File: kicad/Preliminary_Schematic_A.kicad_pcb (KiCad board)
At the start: 2 copper layers, 55.9 x 36.8 mm, 12 parts, among them J1 Input, M1 Motor_Servo, Q1 NMOS, U1 VL53L4CDV0DH/1

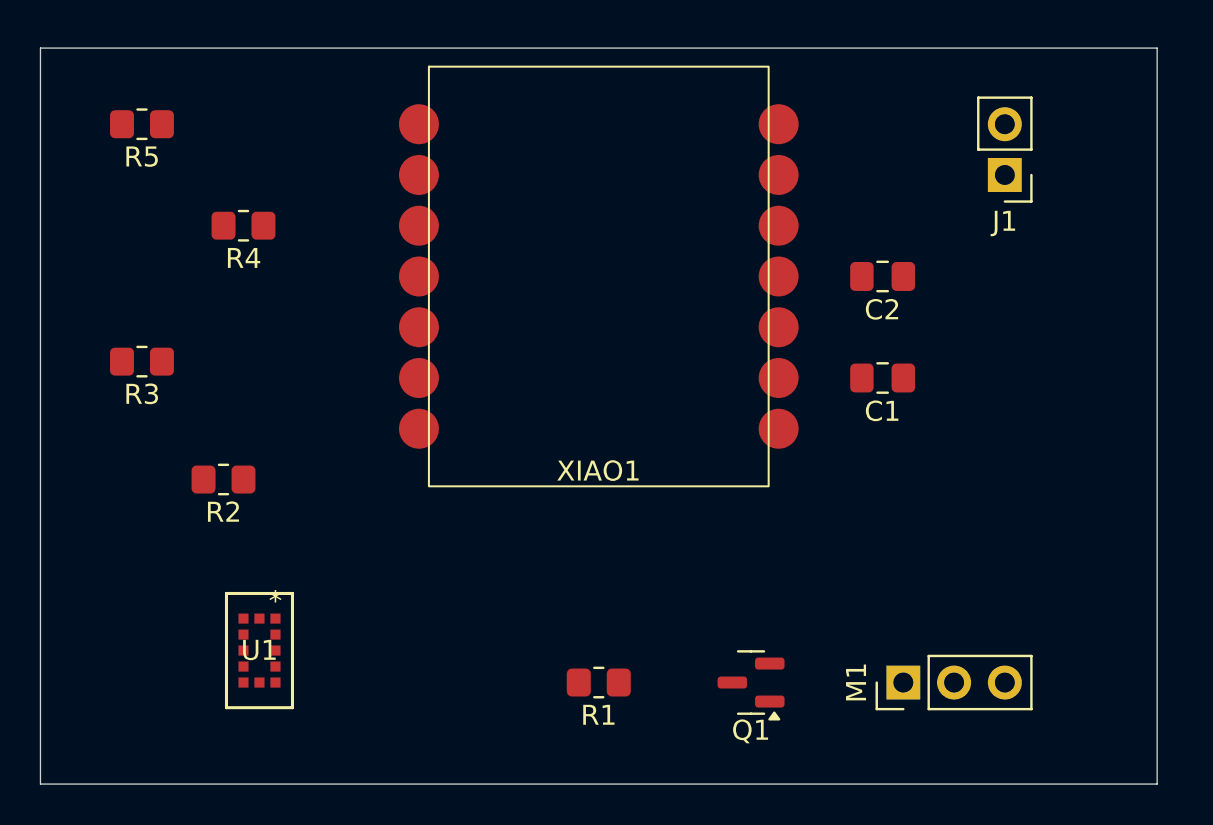
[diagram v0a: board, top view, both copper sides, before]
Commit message: Add files via upload
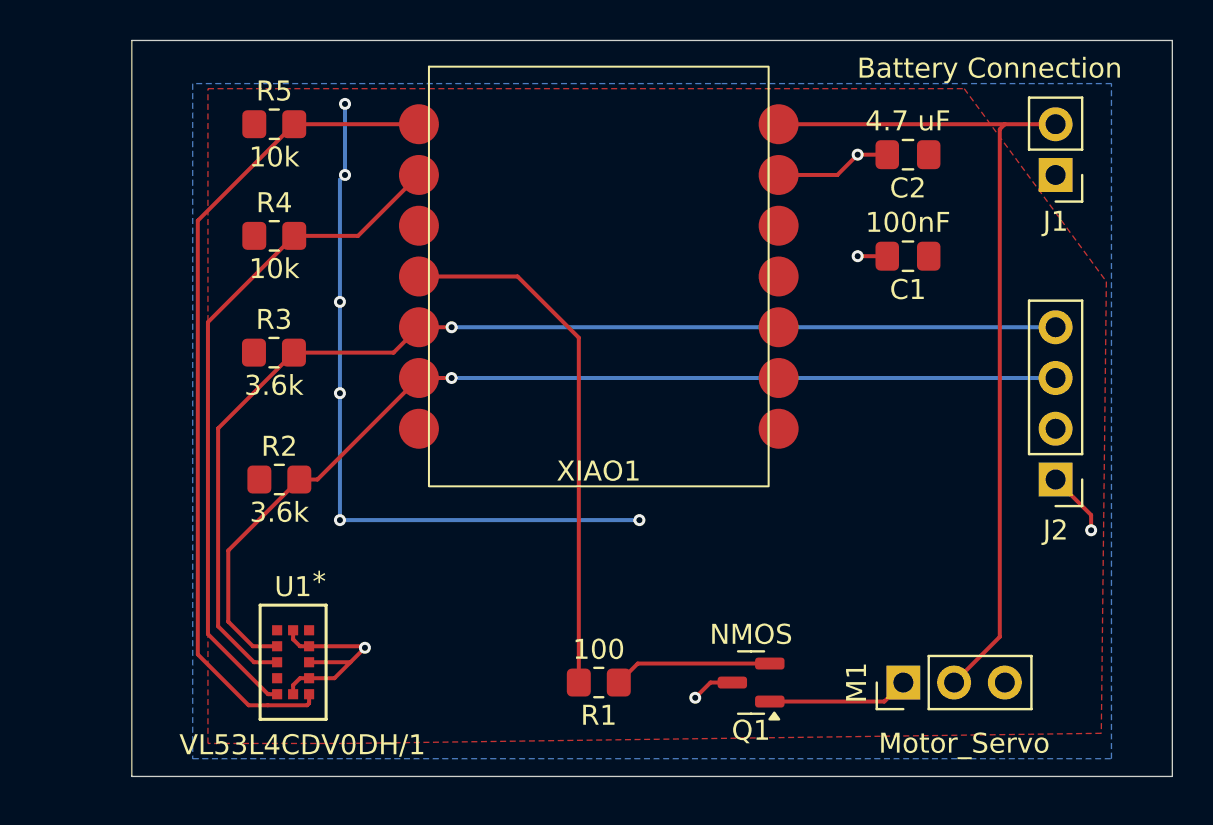
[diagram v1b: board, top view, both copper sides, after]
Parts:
- added J2: Load Cell System, Connector_PinHeader_2.54mm:PinHeader_1x04_P2.54mm_Vertical, F.Cu at (171.4, 108.0)
- J1: value Input -> Battery Connection
- moved R5 6.62 mm to (132.3, 90.2), turned to 0 degrees
- moved R3 6.62 mm to (132.3, 101.6), turned to 0 degrees
- moved C1 6.23 mm to (164.1, 96.8)
- moved C2 6.23 mm to (164.1, 91.7)
- moved R2 2.79 mm to (132.6, 108.0), turned to 0 degrees
- moved J1 2.54 mm to (171.4, 92.7)
- moved U1 1.78 mm to (133.3, 117.1)
- moved R4 1.62 mm to (132.3, 95.8), turned to 0 degrees
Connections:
- net Net-(J1-Pin_1) renamed GND
- R2 pad 1: /3.3V_ESP32 -> /3.3V ESP32
- R3 pad 1: /3.3V_ESP32 -> /3.3V ESP32
- R4 pad 1: /3.3V_ESP32 -> /3.3V ESP32
- R5 pad 1: /3.3V_ESP32 -> /3.3V ESP32
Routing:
- net Net-(J2-Pin_4): track 0.00 -> 57.6 mm, vias 0 -> 1
- net Net-(J2-Pin_3): track 0.00 -> 51.5 mm, vias 0 -> 1
- net Net-(J1-Pin_2): track 0.00 -> 42.9 mm
- net Net-(U1-XSHUT): track 0.00 -> 41.9 mm
- net /3.3V ESP32: track 0.00 -> 35.9 mm, vias 0 -> 6
- net Net-(U1-GPIO1): track 0.00 -> 33.9 mm
- net Net-(R1-Pad2): track 0.00 -> 26.5 mm
- net GND: track 0.00 -> 23.9 mm, vias 0 -> 5
- net Net-(Q1-G): track 0.00 -> 7.95 mm
- net Net-(M1-PWM): track 0.00 -> 7.08 mm
- added copper zone on F.Cu, net /3.3V ESP32
- added copper zone on B.Cu, net GND
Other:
- board size 55.9 x 36.8 mm -> 52.1 x 36.8 mm
